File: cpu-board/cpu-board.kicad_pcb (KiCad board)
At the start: 2 copper layers, 95.5 x 65 mm, 36 parts, among them P1 DATA, P2 ADDR1, P3 ADDR2, P4 CTRL1, P5 CTRL2, P6 PWR, SW1 RESET, U1 WD65C02, U2 AT28C256, U3 MXO45HS, U4 74HC132, U5 CY7C199, U6 4012, U7 4012, U8 74HC138, U9 7805

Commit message: move to biggr PCB for the moment
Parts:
- U9: footprint Discret:TO220_VERT -> Discret:LM78XXV
- moved P3 216.7 mm to (40.1, 83.8), turned to 270 degrees
- moved R7 210.4 mm to (89.9, 140.7)
- moved U7 210.1 mm to (57.4, 105.2), turned to 180 degrees
- moved C10 191.8 mm to (72.6, 103.6)
- moved P2 189.2 mm to (40.1, 61.0), turned to 270 degrees
- moved C9 189.0 mm to (69.6, 103.6), turned to 270 degrees
- moved U6 180.5 mm to (84.3, 105.2)
- moved D1 177.2 mm to (95.5, 131.6), turned to 270 degrees
- moved U9 176.3 mm to (45.2, 116.8), turned to 0 degrees
- moved C5 175.8 mm to (56.4, 119.4), turned to 90 degrees
- moved U2 168.7 mm to (59.9, 76.2), turned to 90 degrees
- moved SW1 166.1 mm to (108.7, 136.7)
- moved U4 165.8 mm to (109.2, 105.2)
- moved C8 165.0 mm to (100.6, 135.6), turned to 90 degrees
- moved P6 157.6 mm to (40.1, 115.3), turned to 270 degrees
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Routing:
- added copper zone on B.Cu, net GND
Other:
- board size 95.5 x 65 mm -> 89.9 x 149.4 mm

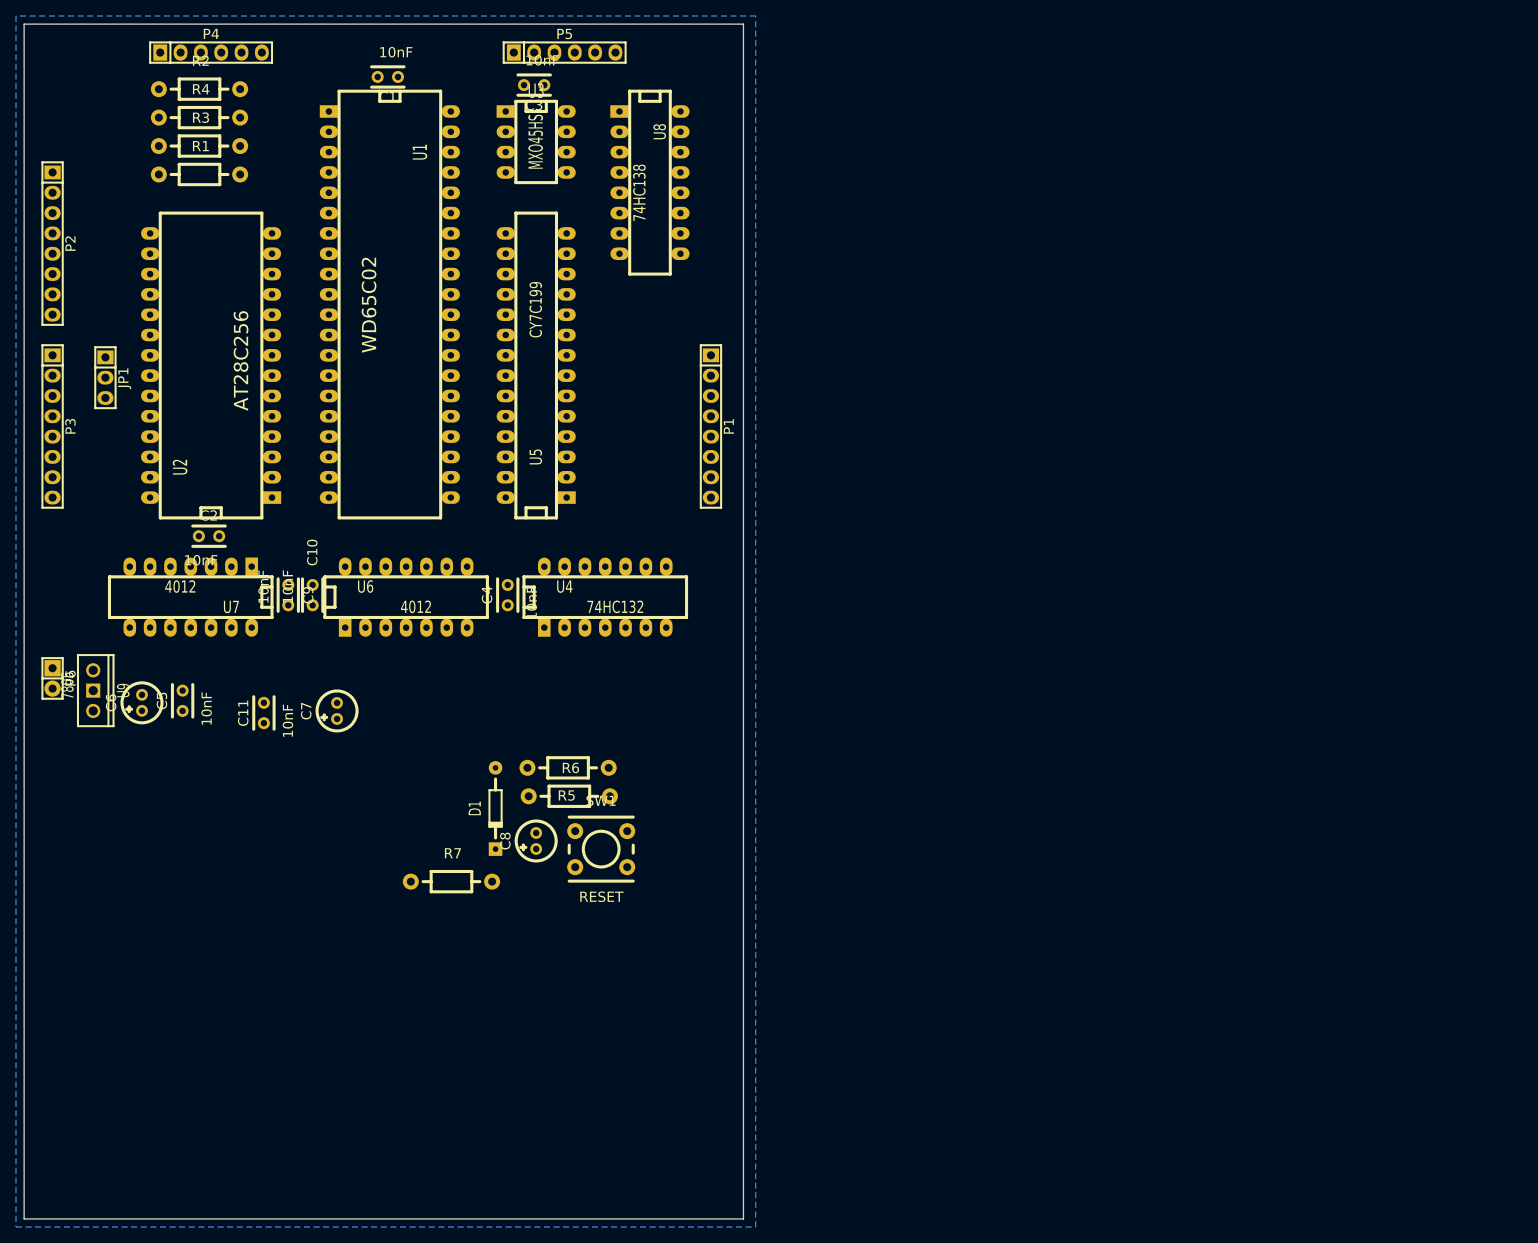
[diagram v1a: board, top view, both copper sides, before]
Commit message: more PCB fiddles
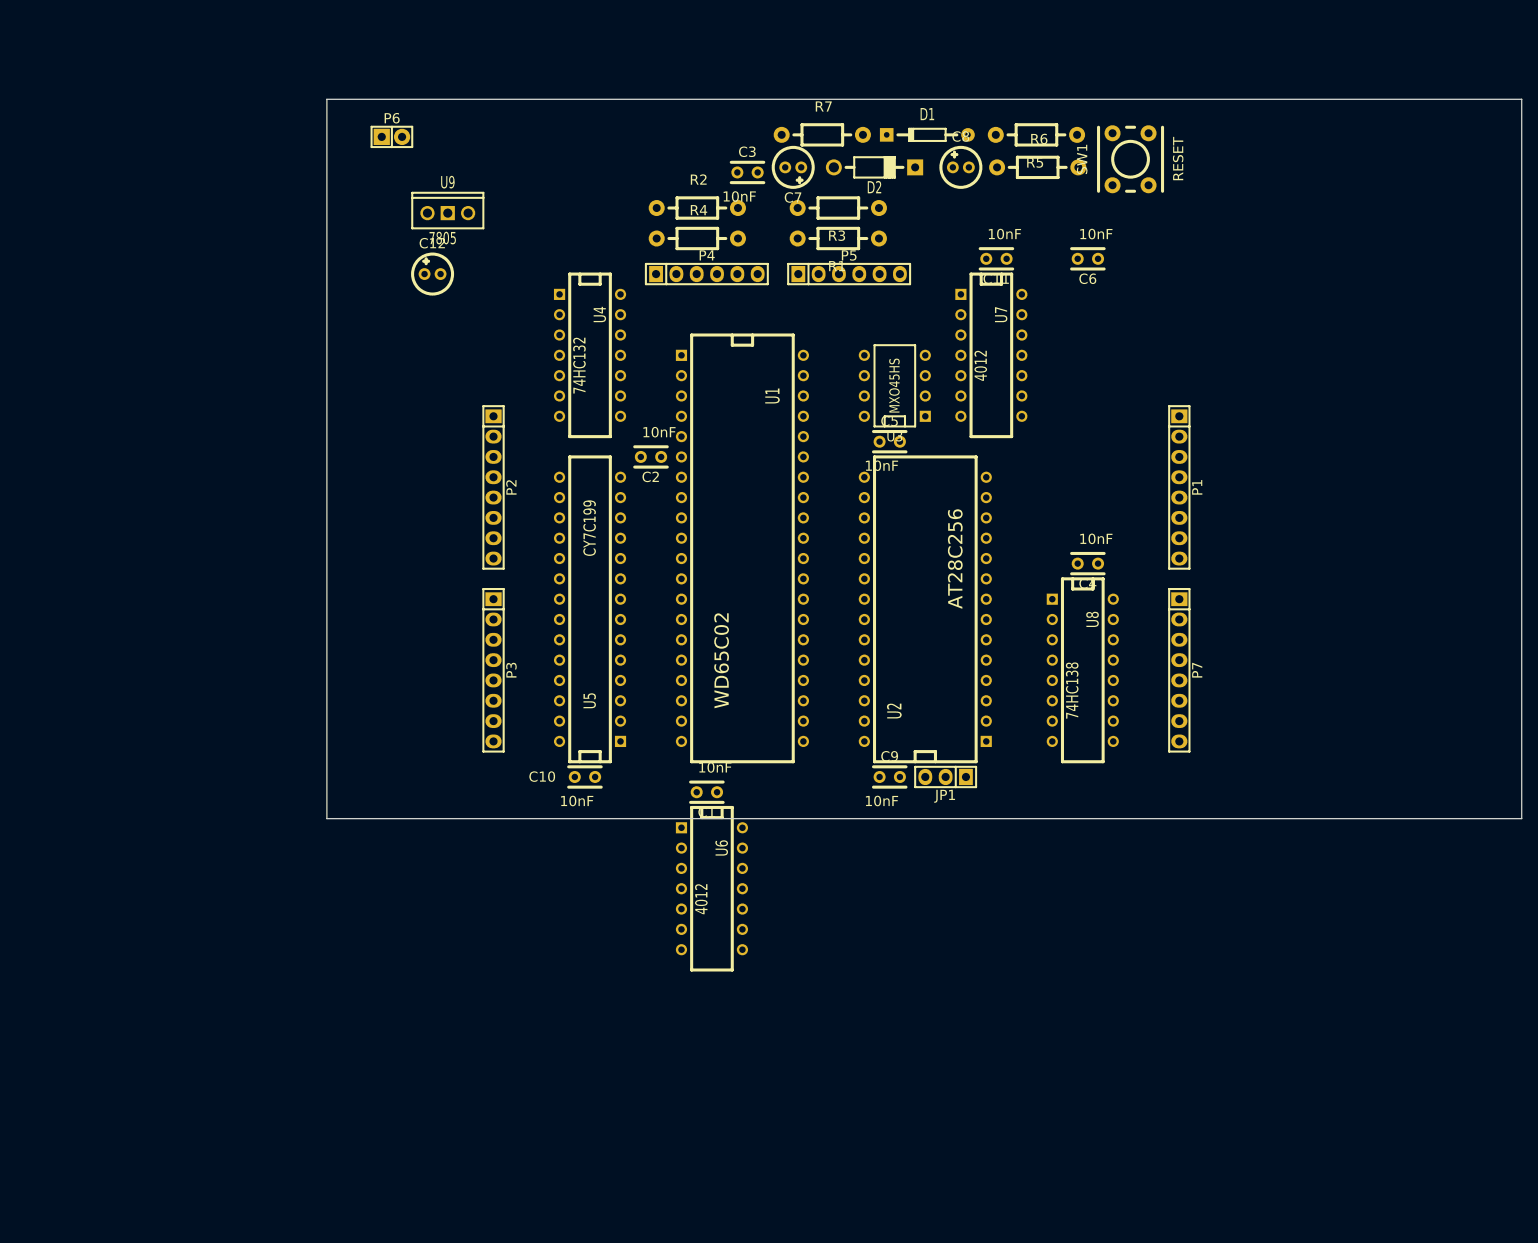
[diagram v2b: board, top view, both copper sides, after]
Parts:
- added C12: 4.7uF, Capacitors_Elko_ThroughHole:Elko_vert_DM5_RM2, F.Cu at (87.6, 64.8)
- added D2: 1N4001, Diodes_ThroughHole:Diode_DO-41_SOD81_Horizontal_RM10, F.Cu at (142.9, 51.4)
- added P7: IO, Socket_Strips:Socket_Strip_Straight_1x08, F.Cu at (181.0, 114.3)
- C6: value 100nF -> 10nF; footprint Capacitors_Elko_ThroughHole:Elko_vert_DM5_RM2 -> Capacitors_ThroughHole:Capacitor4x3RM2.5
- C7: value 100uF -> 4.7uF
- P1, P2, P3: footprint Pin_Headers:Pin_Header_Straight_1x08 -> Socket_Strips:Socket_Strip_Straight_1x08
- P4, P5: footprint Pin_Headers:Pin_Header_Straight_1x06 -> Socket_Strips:Socket_Strip_Straight_1x06
- R1, R2, R3, R4: value 3.3K -> 10K
- U1: footprint Sockets_DIP:DIP-40__600_ELL -> Sockets_DIP:DIP-40__600
- U2: footprint Sockets_DIP:DIP-28__600_ELL -> Sockets_DIP:DIP-28__600
- U3: footprint Sockets_DIP:DIP-8__300_ELL -> Sockets_DIP:DIP-8__300
- U4, U6, U7: footprint Sockets_DIP:DIP-14__300_ELL -> Sockets_DIP:DIP-14__300
- U5: footprint Sockets_DIP:DIP-28__300_ELL -> Sockets_DIP:DIP-28__300
- U8: footprint Sockets_DIP:DIP-16__300_ELL -> Sockets_DIP:DIP-16__300
- moved C6 131.8 mm to (170.8, 62.9), turned to 180 degrees
- moved JP1 116.3 mm to (151.8, 127.6), turned to 180 degrees
- moved C11 109.5 mm to (159.4, 62.9), turned to 180 degrees
- moved SW1 108.7 mm to (174.9, 50.4), turned to 90 degrees
- moved U7 104.5 mm to (157.5, 74.9), turned to 270 degrees
- moved R7 104.2 mm to (136.3, 47.4)
- moved D1 100.0 mm to (149.5, 47.4), turned to 180 degrees
- moved C8 99.5 mm to (153.7, 51.4), turned to 0 degrees
- moved R5 98.4 mm to (163.2, 47.4)
- moved R6 98.0 mm to (163.2, 51.4)
- moved C1 97.9 mm to (123.2, 129.5)
- moved U2 94.3 mm to (149.2, 106.7)
- moved C5 93.4 mm to (143.5, 85.7), turned to 0 degrees
- moved C7 88.7 mm to (132.7, 51.4), turned to 180 degrees
- moved U8 81.5 mm to (168.9, 114.3)
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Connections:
- U8 pad 10: (no net) -> /Address Decode/~IO5
- U8 pad 11: (no net) -> /Address Decode/~IO4
- U8 pad 12: (no net) -> /Address Decode/~IO3
- U8 pad 13: (no net) -> /Address Decode/~IO2
- U8 pad 14: (no net) -> /Address Decode/~IO1
- U8 pad 15: (no net) -> /Address Decode/~IO0
- U8 pad 7: (no net) -> /Address Decode/~IO7
- U8 pad 9: (no net) -> /Address Decode/~IO6
- U9 pad VI: /VIN -> Net-(C12-Pad1)
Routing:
- removed copper zone on B.Cu, net GND
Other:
- board size 89.9 x 149.4 mm -> 149.4 x 89.9 mm
- net class Default: via_dia 0.889 -> 1; via_drill 0.635 -> 0.8
- net class Power added: clearance 0.508, trace_width 0.508, via_dia 1, via_drill 0.8
- rule via_min_drill: 0.508 -> 0.8
- rule via_min_size: 0.889 -> 1
